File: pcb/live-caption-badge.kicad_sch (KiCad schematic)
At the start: 43 parts, among them J2 Conn_01x06, J5 USB_C_Receptacle_USB2.0_16P, Q2 SS8050, Q3 SS8050, SW1 SW_DPDT_x2, SW2 RST, SW3 BTN, SW4 BTN, SW5 BTN, SW6 FLASH, U1 ESP32-S3-WROOM-1, U2 HE9073A33M5R, U3 HE9073A33M5R

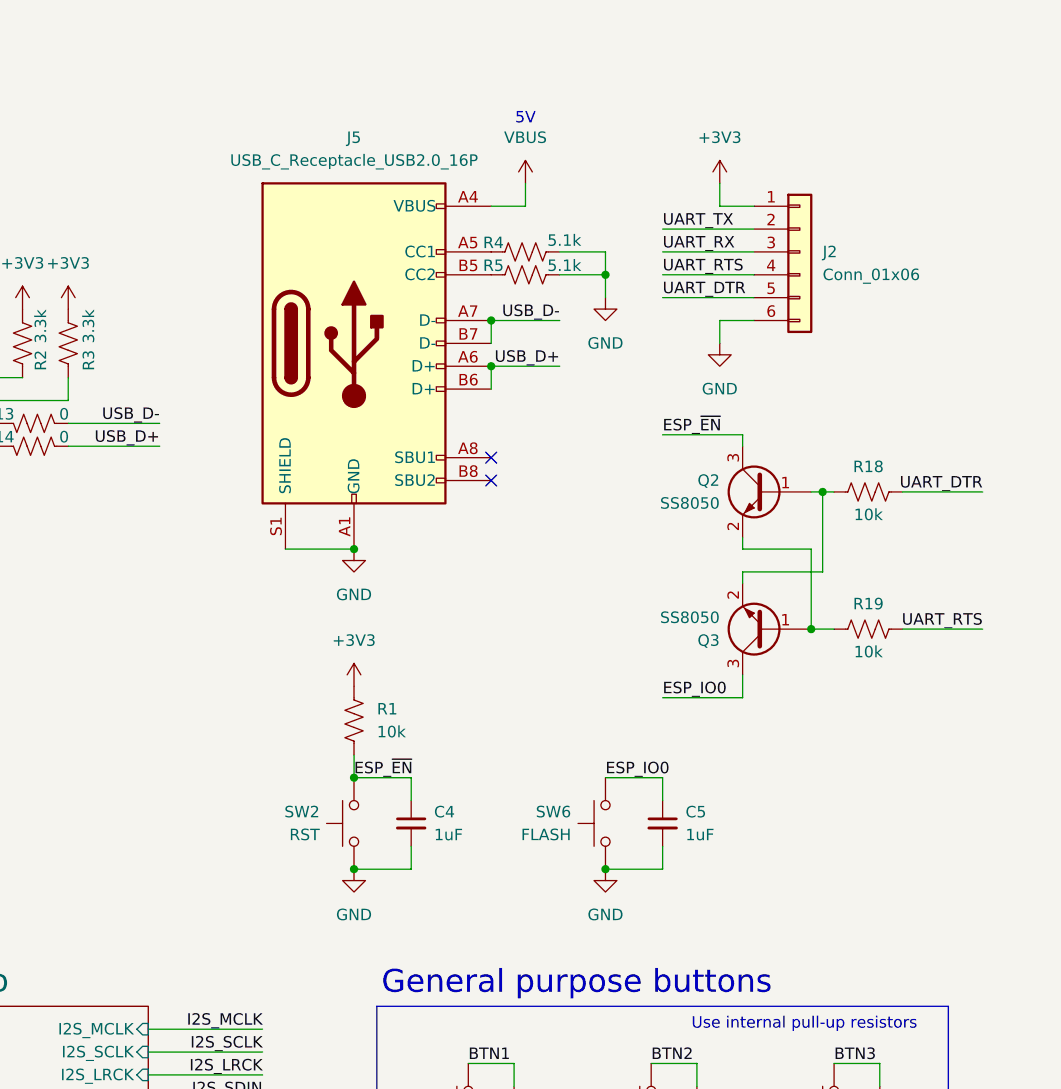
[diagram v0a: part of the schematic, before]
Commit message: pcb: rev 2 ready?
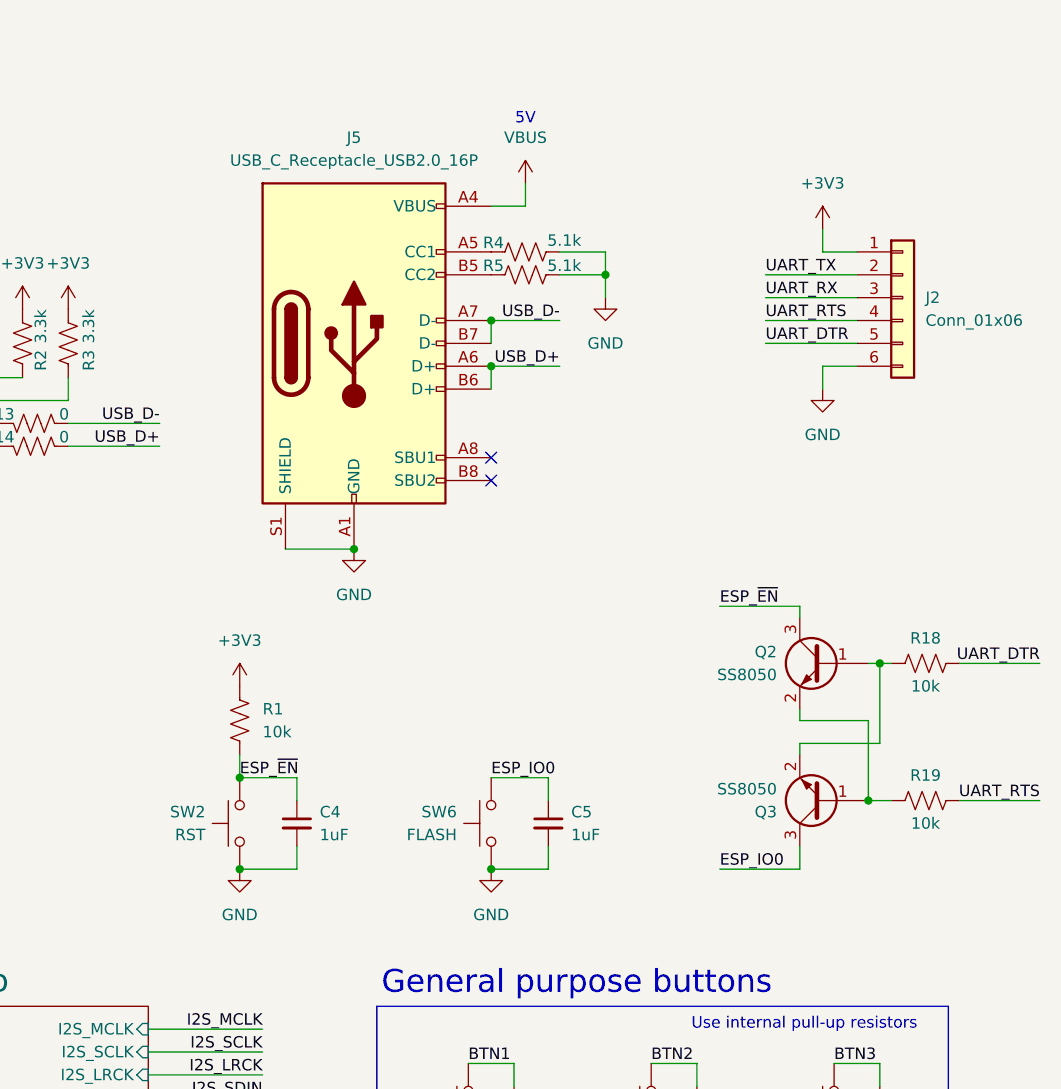
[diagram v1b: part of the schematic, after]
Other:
- moved on the sheet: C4, C5, J2, Q2, Q3, R1, R18, R19, SW2, SW6
